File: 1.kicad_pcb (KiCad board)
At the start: 2 copper layers, 85.1 x 46.4 mm, 44 parts, among them J1 Micro_SD_Card, J10 I2C1, J11 I2C2, J12 B3..9A, J2 USB_B_Micro, J3 Conn_Power, J4 SWD, J5 Protected, J6 SPI1, J7 ADC, J8 UART1, J9 SPI2, K1 NRST, K2 WKUP, K3 KPA0, U1 STM32F103C8Tx, U2 AMS1117-3.3, Y1 8MHz, Y2 32.768k

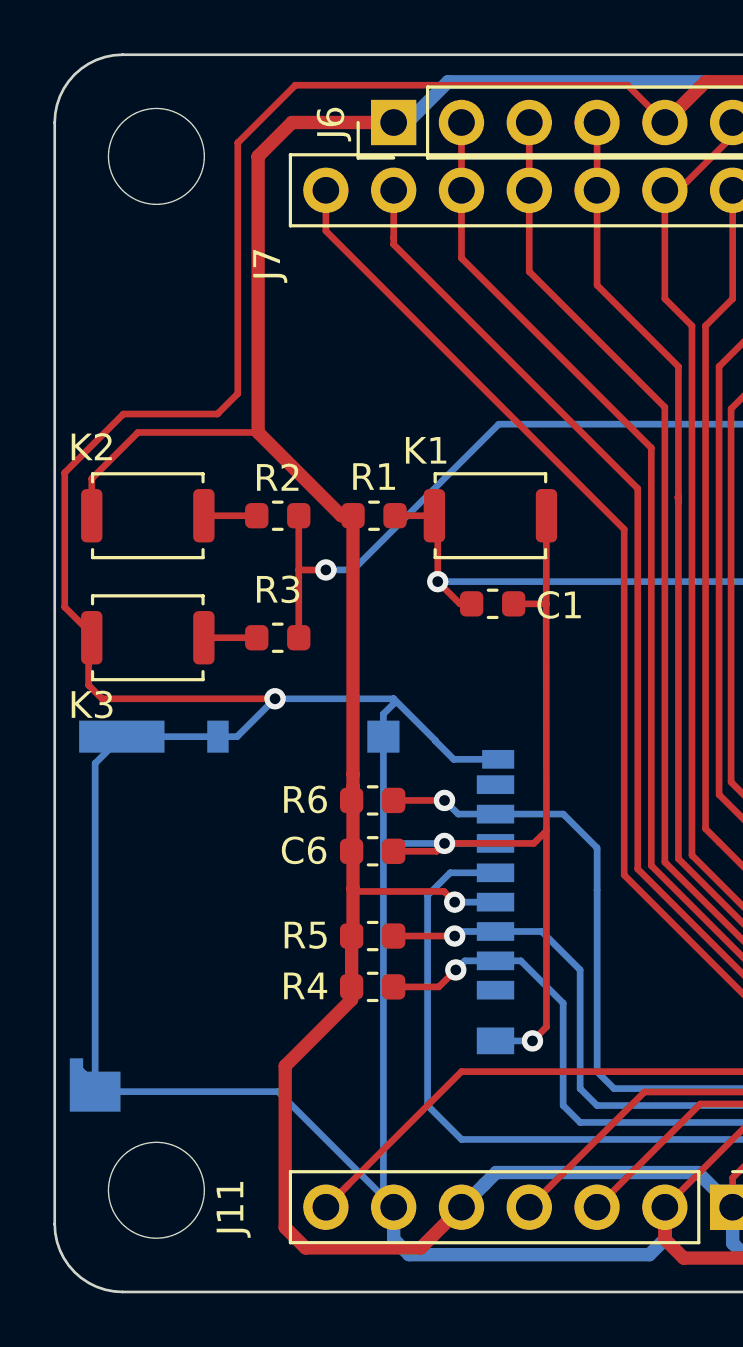
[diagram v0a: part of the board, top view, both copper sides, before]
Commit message: fix lines
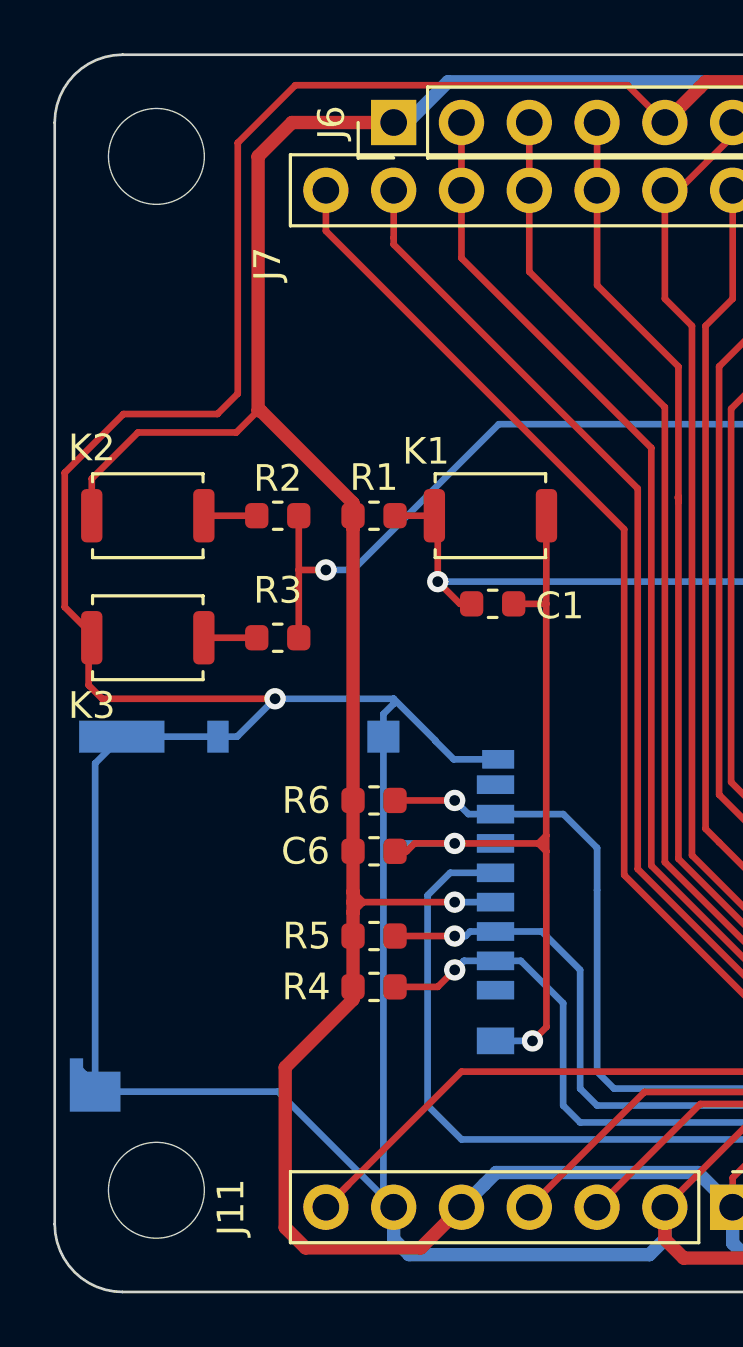
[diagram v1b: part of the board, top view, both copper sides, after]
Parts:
- moved C6 0.05 mm to (108.5, 116.2)
- moved R4 0.05 mm to (108.5, 121.3)
- moved R5 0.05 mm to (108.5, 119.4)
- moved R6 0.05 mm to (108.5, 114.3)
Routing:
- net +3V3: track 290.3 -> 291.7 mm
- net GND: track 554.2 -> 552.9 mm

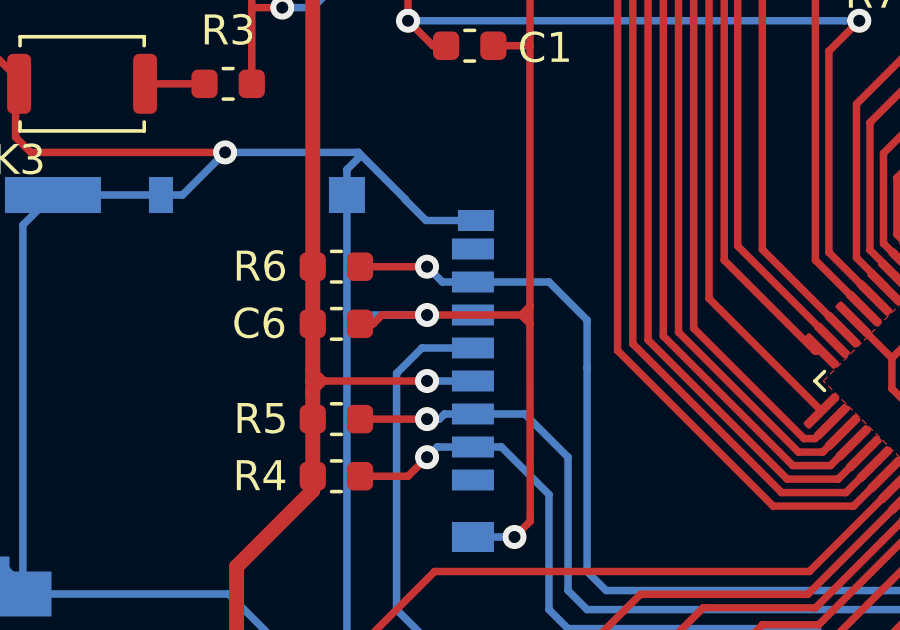
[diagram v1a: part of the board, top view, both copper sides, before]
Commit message: fix lines2
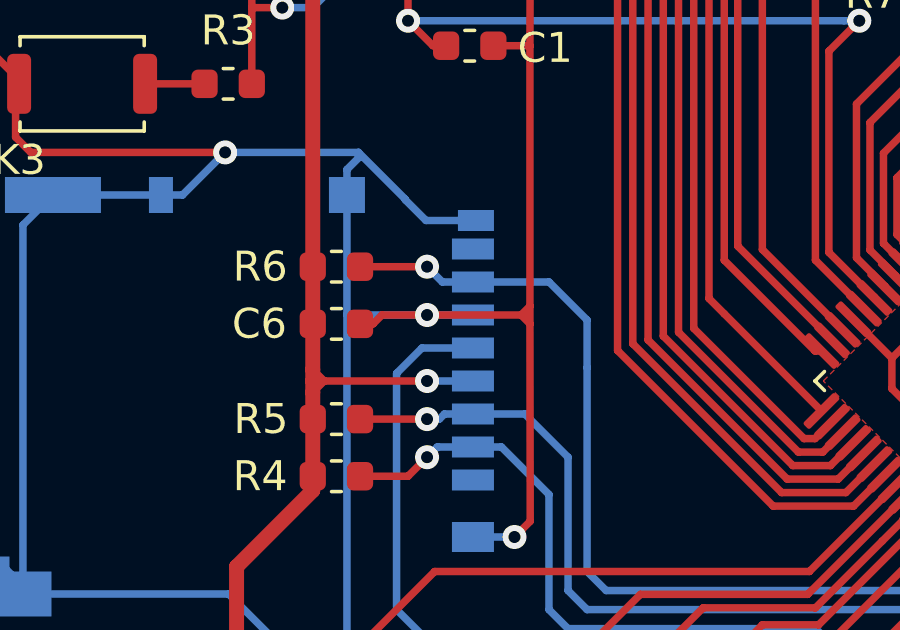
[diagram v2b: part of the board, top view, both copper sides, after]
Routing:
- net GND: track 552.9 -> 554.5 mm
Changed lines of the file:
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@@
     (thickness 1.6)
     (drawings 44)
-    (tracks 674)
+    (tracks 675)
     (zones 0)
     (modules 44)
@@
   (segment (start 111.506 115.91) (end 108.8408 115.91) (width 0.25) (layer B.Cu) (net 7))
   (segment (start 108.835 111.91) (end 108.835 115.9042) (width 0.25) (layer B.Cu) (net 7))
+  (segment (start 111.506 115.91) (end 113.035 115.91) (width 0.25) (layer B.Cu) (net 7))
   (segment (start 163.83 100.838) (end 170.18 100.838) (width 0.25) (layer F.Cu) (net 8))
   (segment (start 170.18 100.838) (end 170.18 107.95) (width 0.5) (layer F.Cu) (net 8))
